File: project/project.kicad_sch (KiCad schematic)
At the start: 22 parts, among them U2 NE555P, U4 ROB-14450

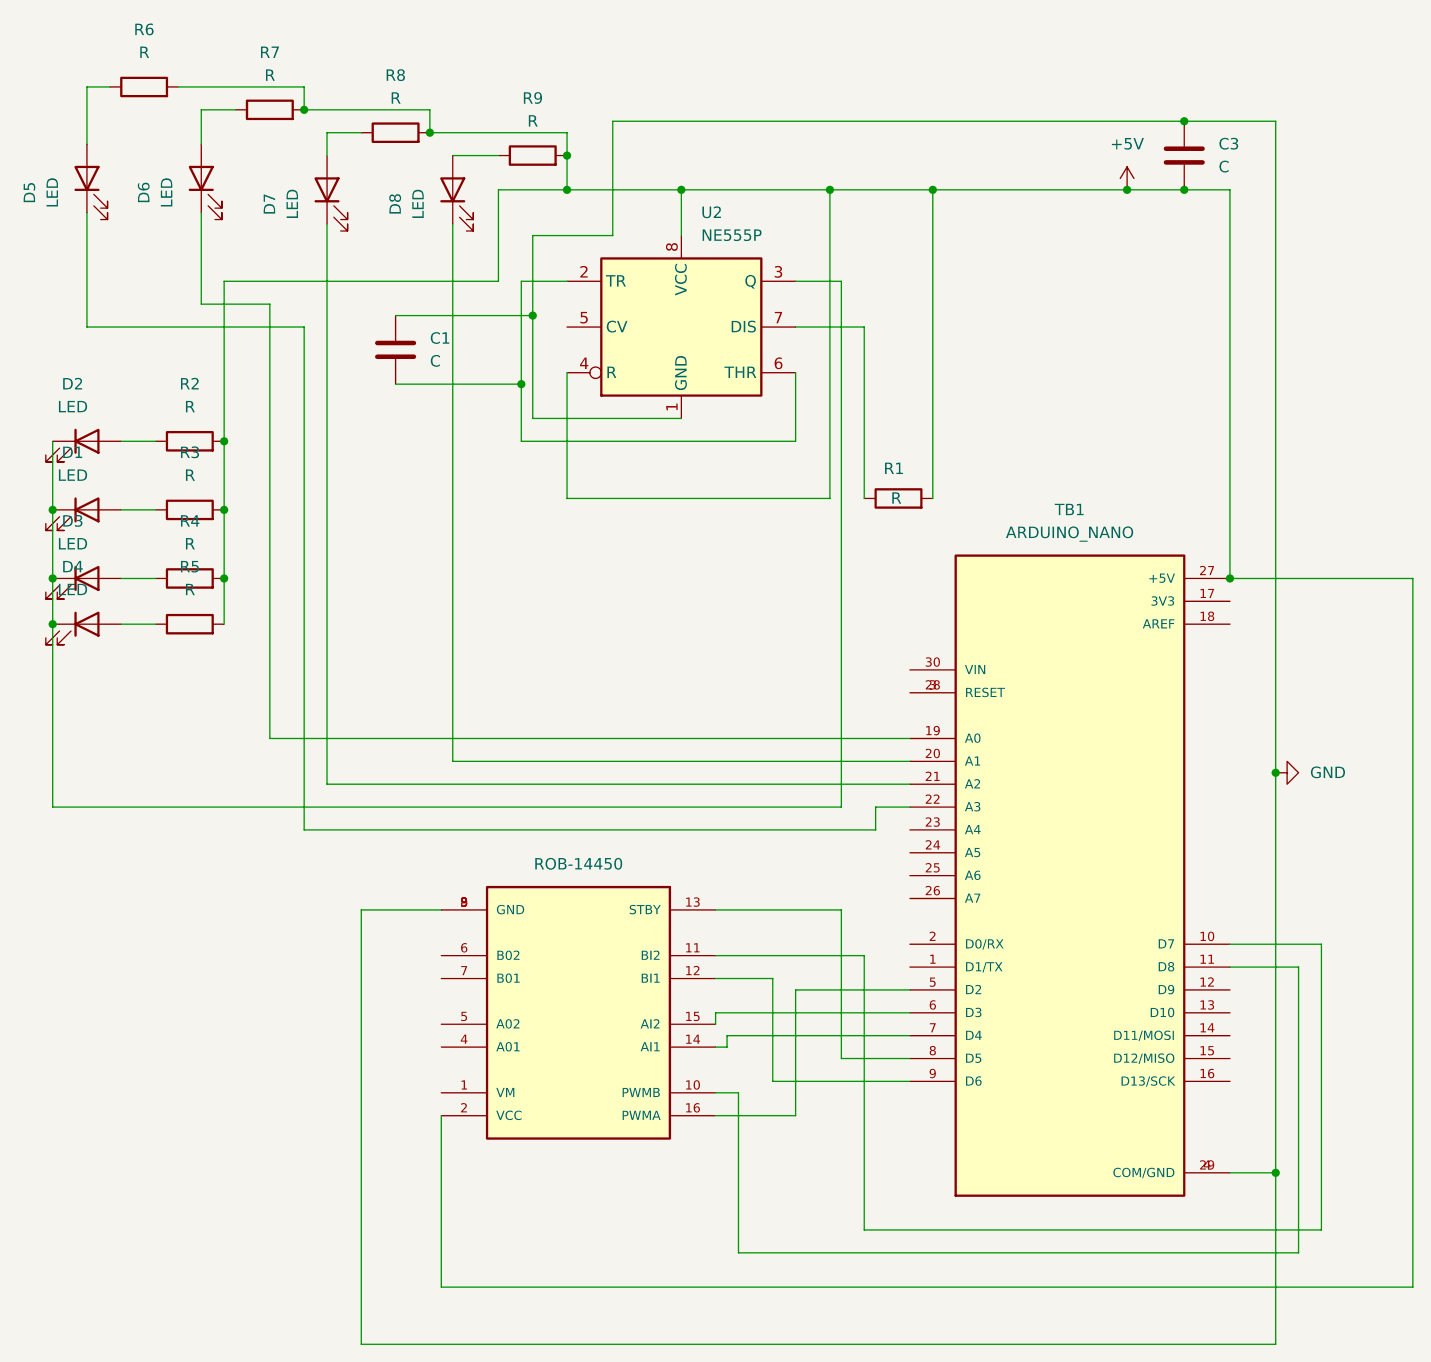
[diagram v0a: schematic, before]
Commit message: Add files via upload
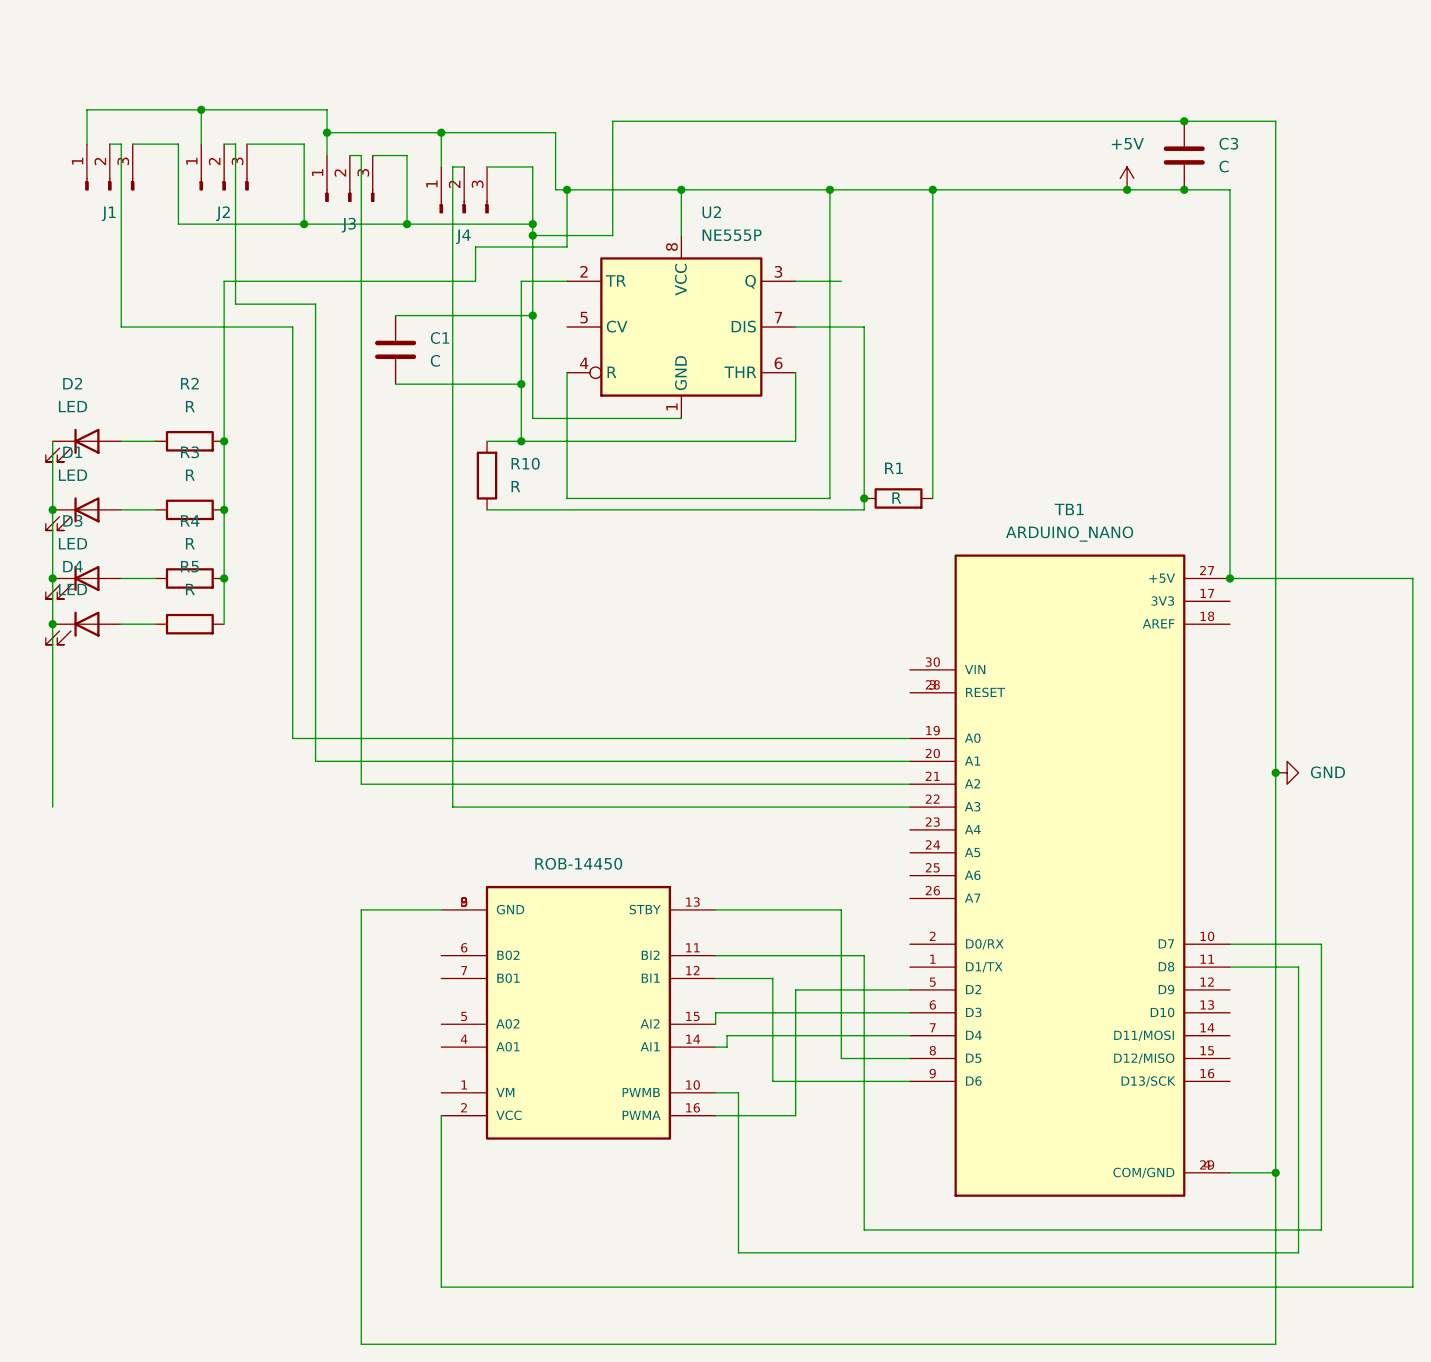
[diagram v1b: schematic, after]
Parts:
- removed D5, D6, D7, D8: LED, LED_THT:LED_D5.0mm, symbol Device:LED
- removed R6, R7, R8, R9: R, Resistor_SMD:R_0805_2012Metric, symbol Device:R
- added J1, J2, J3, J4: Conn_01x03_Pin, Connector_PinSocket_2.00mm:PinSocket_1x03_P2.00mm_Vertical, symbol Connector:Conn_01x03_Pin
- added R10: R, Resistor_SMD:R_0805_2012Metric, symbol Device:R
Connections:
- net +5V: now also J1.1 (Pin_1), J2.1 (Pin_1), J3.1 (Pin_1), J4.1 (Pin_1)
- net GND: now also J1.3 (Pin_3), J2.3 (Pin_3), J3.3 (Pin_3), J4.3 (Pin_3)
- net at TB1.19 (A0): now also J1.2 (Pin_2)
- net at TB1.20 (A1): now also J2.2 (Pin_2)
- net at TB1.21 (A2): now also J3.2 (Pin_2)
- net at TB1.22 (A3): now also J4.2 (Pin_2)
- net at C1.1, U2.2 (TR), U2.6 (THR): now also R10.2
- net at D1.1 (K), D2.1 (K), D3.1 (K)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: no longer U2.3 (Q)
- net at R1.1, U2.7 (DIS): now also R10.1
